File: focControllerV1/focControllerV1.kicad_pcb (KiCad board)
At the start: 2 copper layers, 86.8 x 49 mm, 95 parts, among them J1 Conn_01x05, J2 Conn_01x05, J3 USB_C_Receptacle_USB2.0, Q1 BC818W, Q2 BC818W, SW1 SW_Push, U1 LP2992IM5X-5.0/NOPB, U10 DRV8313PWP, U11 INA240A2PW, U12 INA240A2PW, U13 INA240A2PW, U14 KF301-5.0-2P, U15 ESP32-WROOM-32, U2 ME3116AM6G, U3 DRV8313PWP, U4 INA240A2PW, U5 MPU-6050, U7 CH340C, U8 KF301-5.0-3P, U9 KF301-5.0-3P

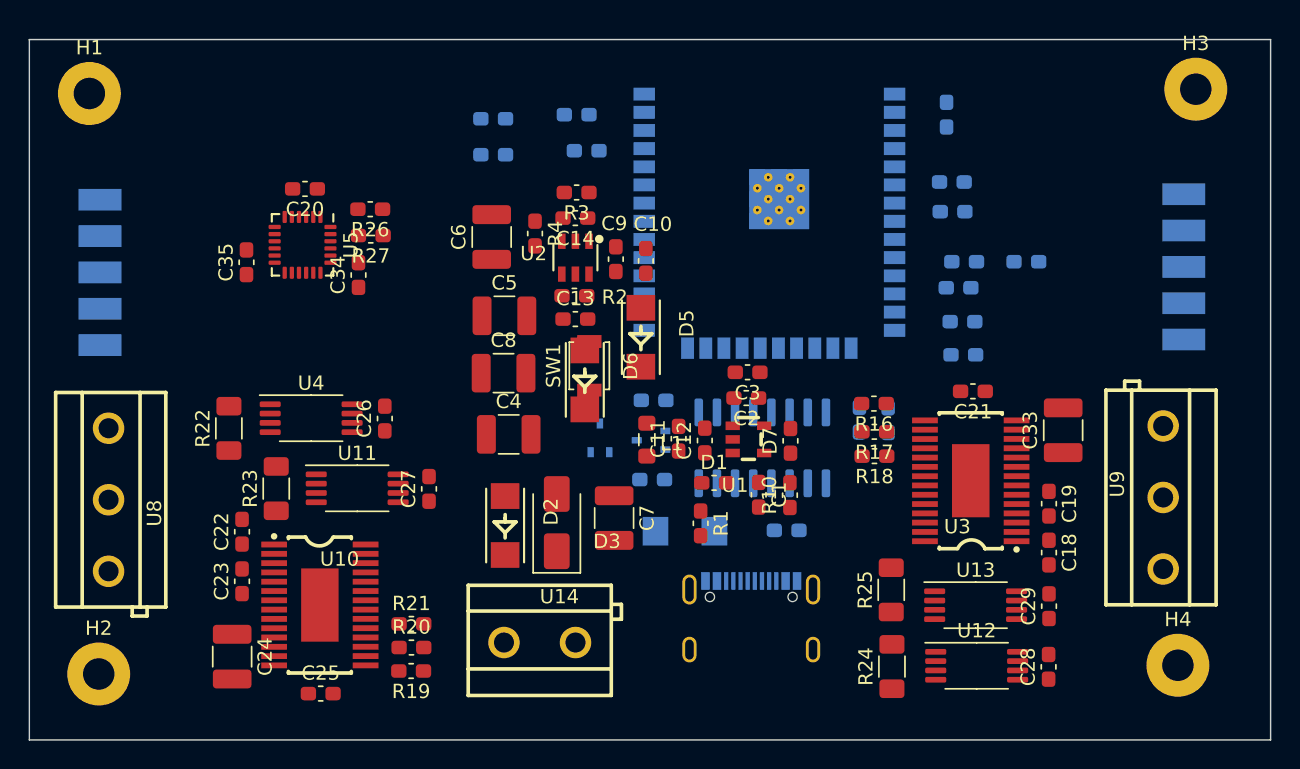
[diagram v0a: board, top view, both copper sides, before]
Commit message: 728
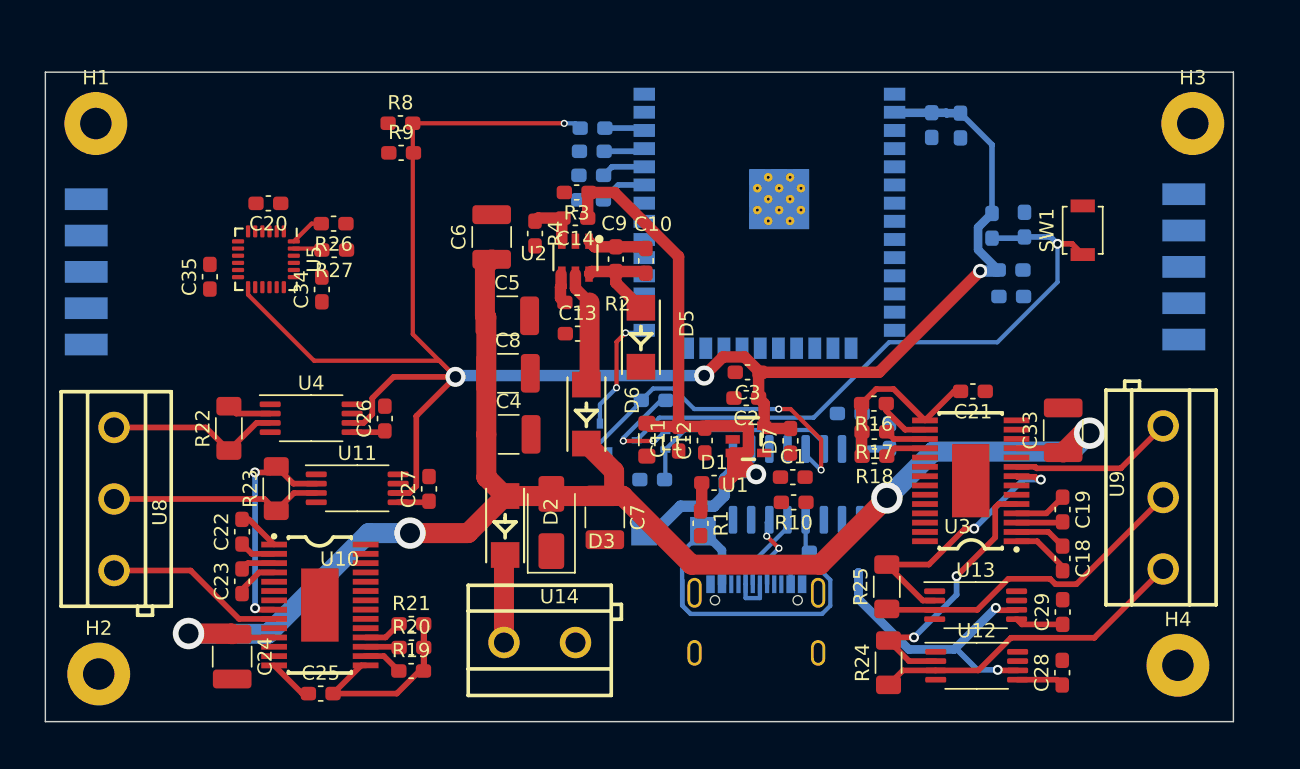
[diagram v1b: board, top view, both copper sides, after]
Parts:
- R8, R9: moved to F.Cu
- moved R9 38.8 mm to (62.7, 71.2), turned to 0 degrees
- moved R8 38.8 mm to (62.7, 69.1), turned to 0 degrees
- moved SW1 35.8 mm to (110.4, 76.6)
- moved C32 32.7 mm to (101.8, 69.3), turned to -90 degrees
- moved C31 30.7 mm to (99.8, 69.2), turned to -90 degrees
- moved R14 29.2 mm to (76.1, 69.5)
- moved R13 28.2 mm to (76.0, 74.5)
- moved C30 9.42 mm to (106.3, 76.2)
- moved R12 3.73 mm to (105.4, 81.2), turned to 0 degrees
- moved U7 3.50 mm to (90.4, 94.4)
- moved R11 3.18 mm to (104.0, 76.3), turned to -90 degrees
- moved C15 2.89 mm to (92.1, 99.1)
- moved R6 2.77 mm to (76.1, 71.1), turned to 0 degrees
- moved C35 2.75 mm to (49.4, 79.8)
- moved U5 2.75 mm to (53.3, 78.6)
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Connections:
- R12 pad 1: unconnected-(R12-Pad1) -> /LED
- U15 pad 30: unconnected-(U15-IO18-Pad30) -> /I2C1_SCL
- U15 pad 31: unconnected-(U15-IO19-Pad31) -> /I2C1_SDA
- U15 pad 33: unconnected-(U15-IO21-Pad33) -> /I2C2_SCL
- U15 pad 36: unconnected-(U15-IO22-Pad36) -> /I2C2_SDA
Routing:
- net +3V3: track 0.00 -> 164.1 mm, vias 0 -> 6
- net VCC: track 0.00 -> 106.5 mm, vias 0 -> 4
- net +5V: track 0.00 -> 51.6 mm, vias 0 -> 1
- net /EN: track 0.00 -> 43.6 mm, vias 0 -> 1
- net Net-(D9-A): track 0.00 -> 32.3 mm
- net /DTR: track 0.00 -> 23.5 mm, vias 0 -> 2
- net /M2_OUT2_N: track 0.00 -> 22.9 mm
- net /M2_OUT1_N: track 0.00 -> 22.6 mm
- net /M2_OUT2_P: track 0.00 -> 19.4 mm, vias 0 -> 2
- net /M2_OUT1_P: track 0.00 -> 18.8 mm, vias 0 -> 2
- net Net-(U10-V3P3OUT): track 0.00 -> 16.5 mm
- net /M1_OUT2_P: track 0.00 -> 15.8 mm, vias 0 -> 2
- net /M1_OUT2_N: track 0.00 -> 15.0 mm
- net /RTS: track 0.00 -> 14.6 mm
- net Net-(U3-V3P3OUT): track 0.00 -> 12.8 mm
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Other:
- board size 86.8 x 49 mm -> 83.1 x 45.4 mm
